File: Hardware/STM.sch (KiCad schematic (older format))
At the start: 19 parts, among them U1 STM32F042K6Tx

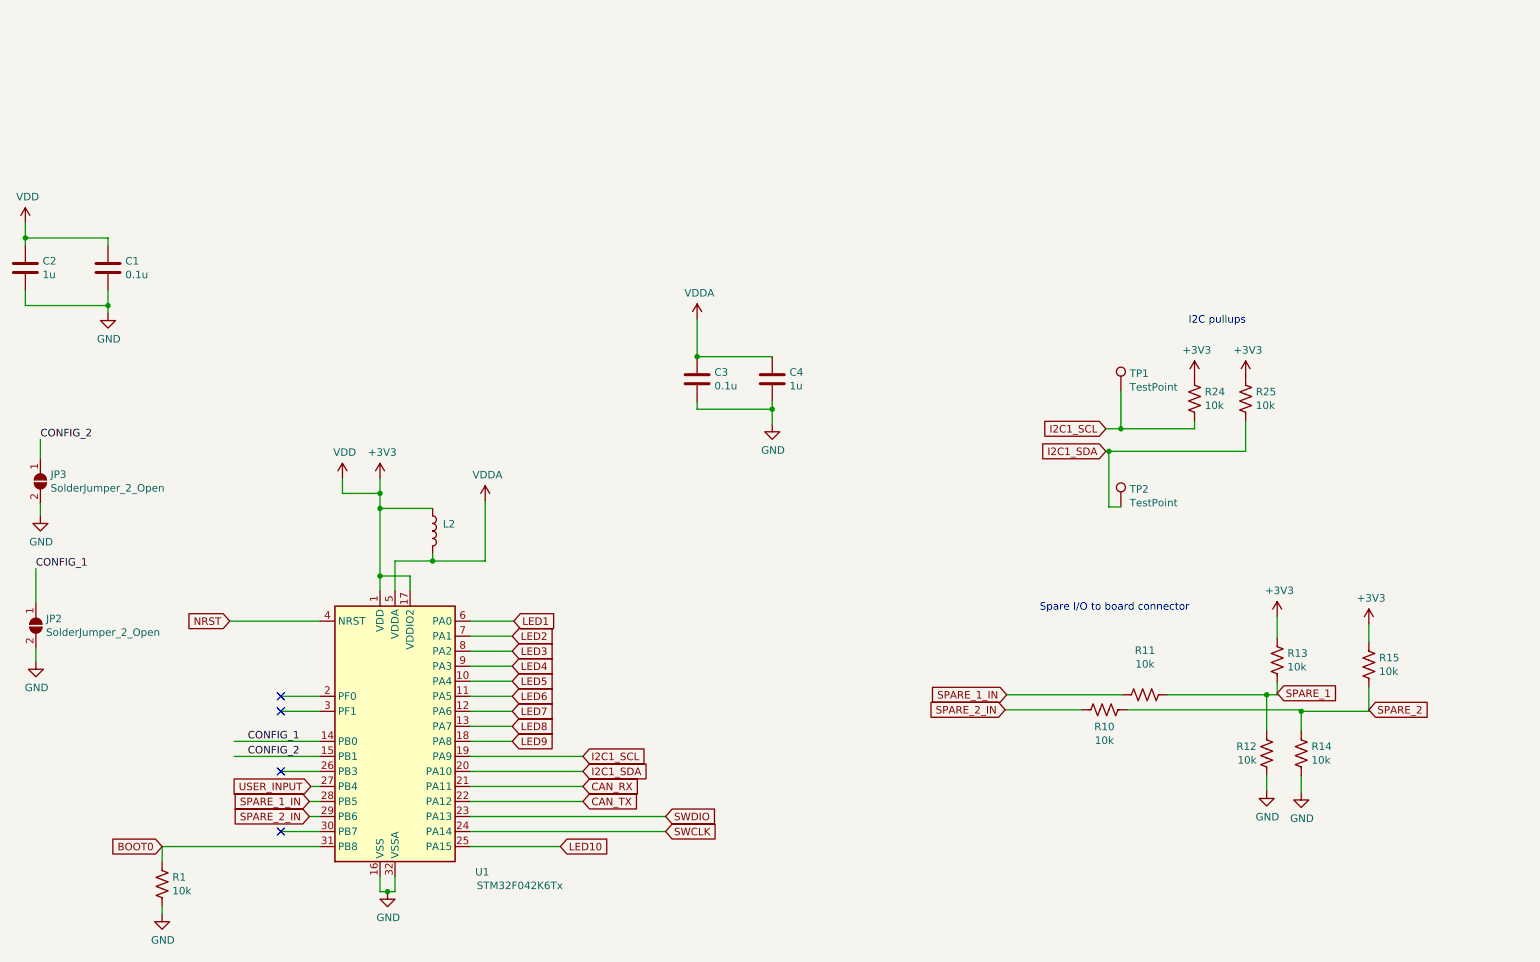
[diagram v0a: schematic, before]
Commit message: Update for F103
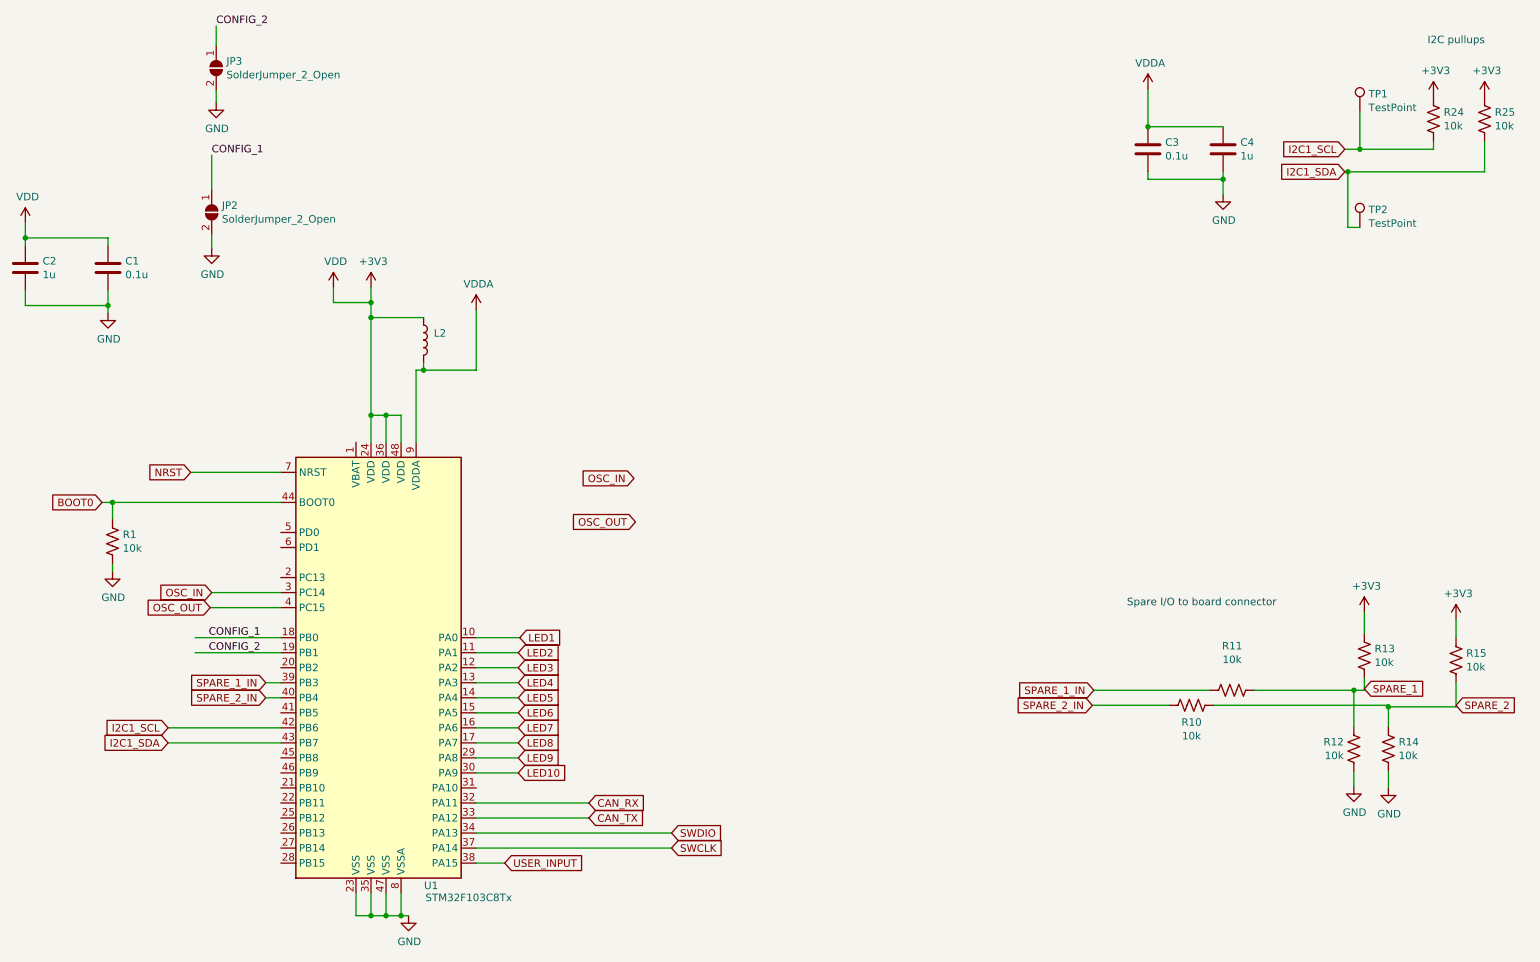
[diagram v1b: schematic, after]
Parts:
- removed U1: STM32F042K6Tx, Package_QFP:LQFP-32_7x7mm_P0.8mm, symbol MCU_ST_STM32F0:STM32F042K6Tx
- added U1: STM32F103C8Tx, Package_QFP:LQFP-48_7x7mm_P0.5mm, symbol MCU_ST_STM32F1:STM32F103C8Tx
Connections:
- net +3V3: now also U1.24 (VDD), U1.36 (VDD), U1.48 (VDD)
- net BOOT0: now also U1.44 (BOOT0)
- net CAN_RX: now also U1.32 (PA11)
- net CAN_TX: now also U1.33 (PA12)
- net CONFIG_1: now also U1.18 (PB0)
- net CONFIG_2: now also U1.19 (PB1)
- net GND: now also U1.23 (VSS), U1.35 (VSS), U1.47 (VSS), U1.8 (VSSA)
- net I2C1_SCL: now also U1.42 (PB6)
- net I2C1_SDA: now also U1.43 (PB7)
- net LED1: now also U1.10 (PA0)
- net LED10: now also U1.30 (PA9)
- net LED2: now also U1.11 (PA1)
- net LED3: now also U1.12 (PA2)
- net LED4: now also U1.13 (PA3)
- net LED5: now also U1.14 (PA4)
- net LED6: now also U1.15 (PA5)
- net LED7: now also U1.16 (PA6)
- net LED8: now also U1.17 (PA7)
- net LED9: now also U1.29 (PA8)
- net NRST: now also U1.7 (NRST)
- net SPARE_1_IN: now also U1.39 (PB3)
- net SPARE_2_IN: now also U1.40 (PB4)
- net SWCLK: now also U1.37 (PA14)
- net SWDIO: now also U1.34 (PA13)
- net USER_INPUT: now also U1.38 (PA15)
- net VDDA: now also U1.9 (VDDA)
- new net OSC_IN: U1.3 (PC14)
- new net OSC_OUT: U1.4 (PC15)
- no-connect marks 4 -> 0
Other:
- moved on the sheet: C3, C4, JP2, JP3, L2, R1, R10, R11, R12, R13, R14, R15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
